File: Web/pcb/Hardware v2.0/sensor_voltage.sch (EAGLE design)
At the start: 18 parts, among them IC1 OPA344, IC2 SI8920BCSMD, J1 22-27-2041-04

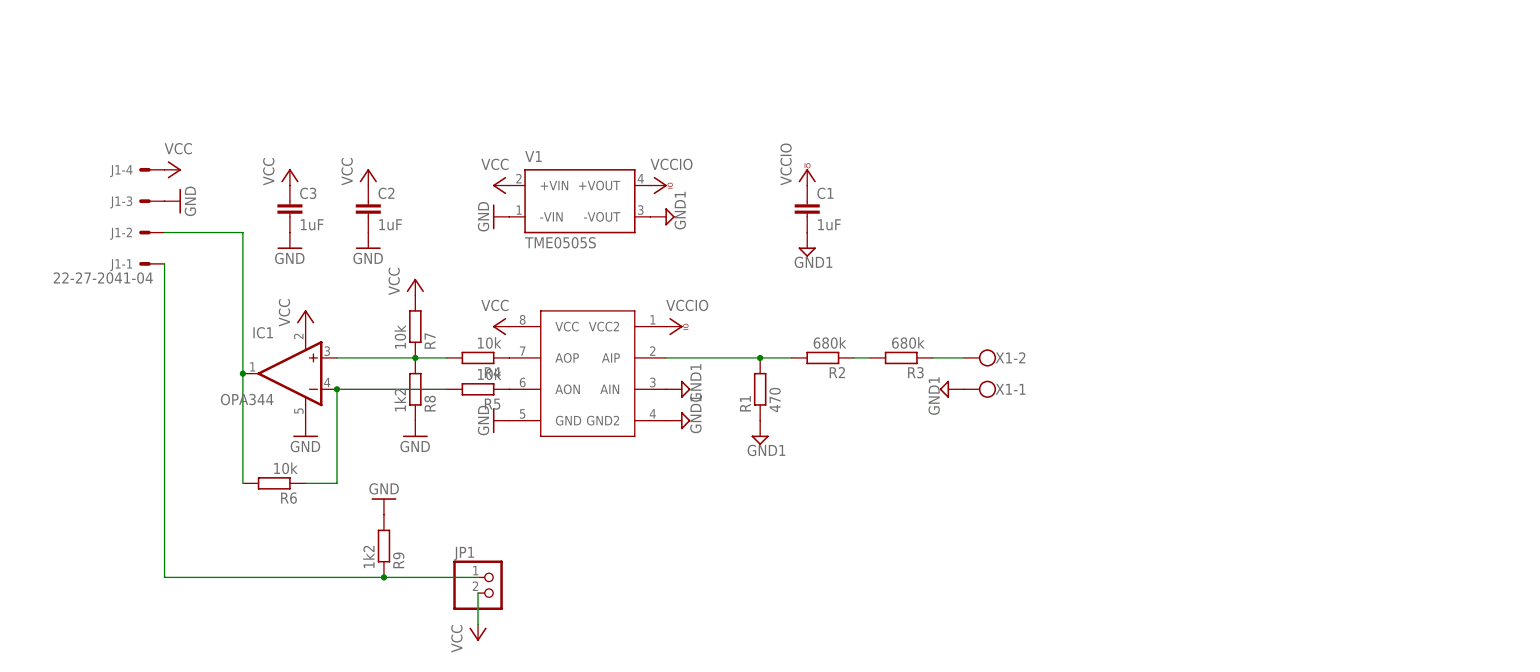
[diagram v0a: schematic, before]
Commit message: updates
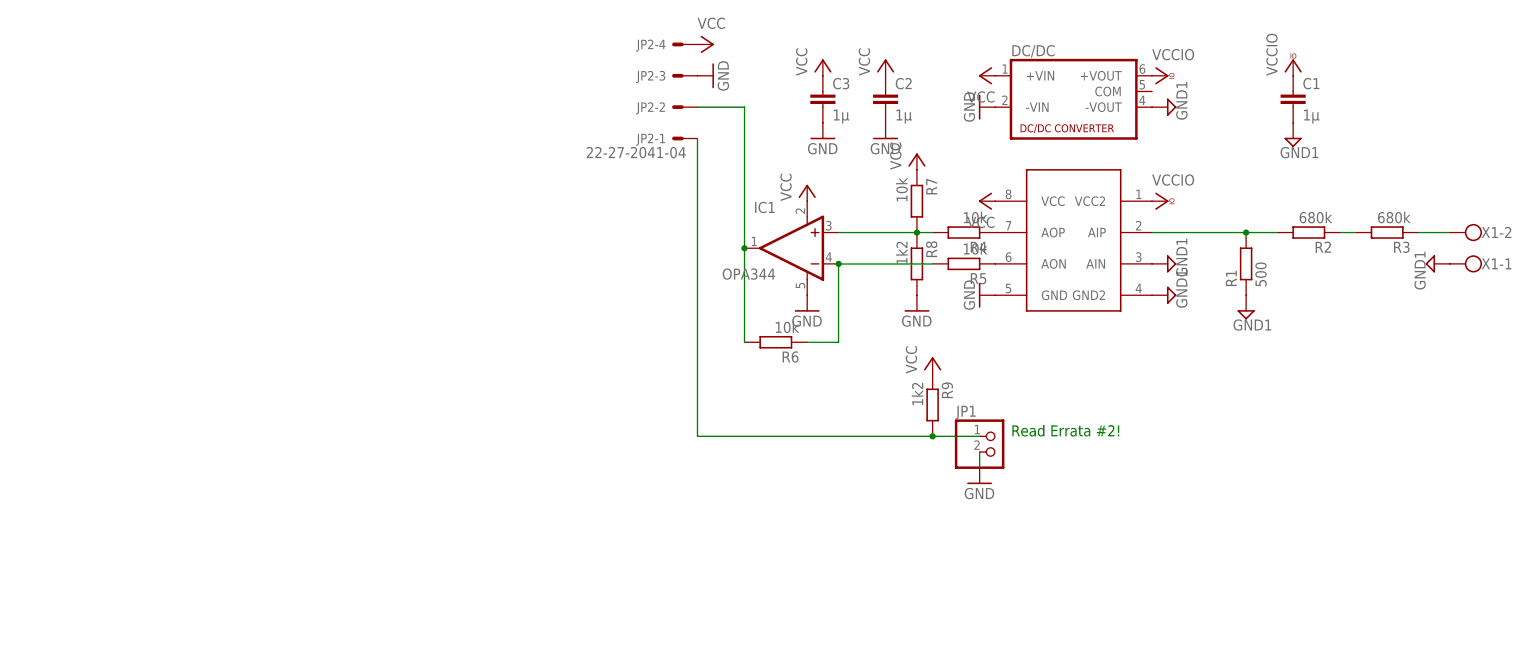
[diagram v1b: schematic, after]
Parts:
- removed J1: 22-27-2041-04, con-molex:22-27-2041-04
- removed V1: TME0505S, traco-electronic:TME0505S
- added DC/DC: (no value), dc-dc-converter:MEV3
- added JP2: 22-27-2041-04, con-molex:22-27-2041-04
- C1, C2, C3: value 1uF -> 1µ
- IC1: device OPA344:OPA344 -> SparkFun-AnalogIC:OPA344
- IC2: value SI8920BCSMD -> SI8920; device SI8920BC:SI8920BCSMD -> silabs:SI8920
- R1: value 470 -> 500; device rcl:R-EU_0309/12 -> rcl:R-EU_0207/10
- R2, R3, R4, R5, R6, R7, R8, R9: device rcl:R-EU_0309/12 -> rcl:R-EU_0207/10
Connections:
- removed net N$3 (its old number): IC1.OUT, J1-2.S, R6.2
- removed net N$4 (its old number): IC1.+IN, R4.2, R7.1, R8.2
- removed net N$5 (its old number): J1-1.S, JP1.1, R9.1
- new net N$6: IC1.OUT, JP2-2.S, R6.2
- new net N$8: IC1.+IN, R4.2, R7.2, R8.1
- new net N$9: JP1.1, JP2-1.S, R9.2
- net GND: now also DC/DC.-VIN, JP1.2, JP2-3.S, R8.2; no longer J1-3.S, R8.1, R9.2, V1.-VIN
- net GND1: now also DC/DC.-VOUT; no longer V1.-VOUT
- net VCC: now also DC/DC.+VIN, JP2-4.S, R7.1, R9.1; no longer J1-4.S, JP1.2, R7.2, V1.+VIN
- net VCCIO: now also DC/DC.+VOUT; no longer V1.+VOUT
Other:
- note added: "Read Errata #2!"
- moved on the sheet: C1, C2, C3, IC1, JP1, R1, R2, R3, R4, R5, R6, R7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
